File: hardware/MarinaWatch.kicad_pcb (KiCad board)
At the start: 2 copper layers, 82.5 x 100.3 mm, 54 parts, among them J201 USB_C_Receptacle_USB2.0_16P, J401 Screw_Terminal_01x04, J801 Screw_Terminal_01x02, J802 Screw_Terminal_01x03, J803 Screw_Terminal_01x03, U101 ESP32-S3-MINI-1, U301 LMV321, U302 LMV321, U303 LMV321

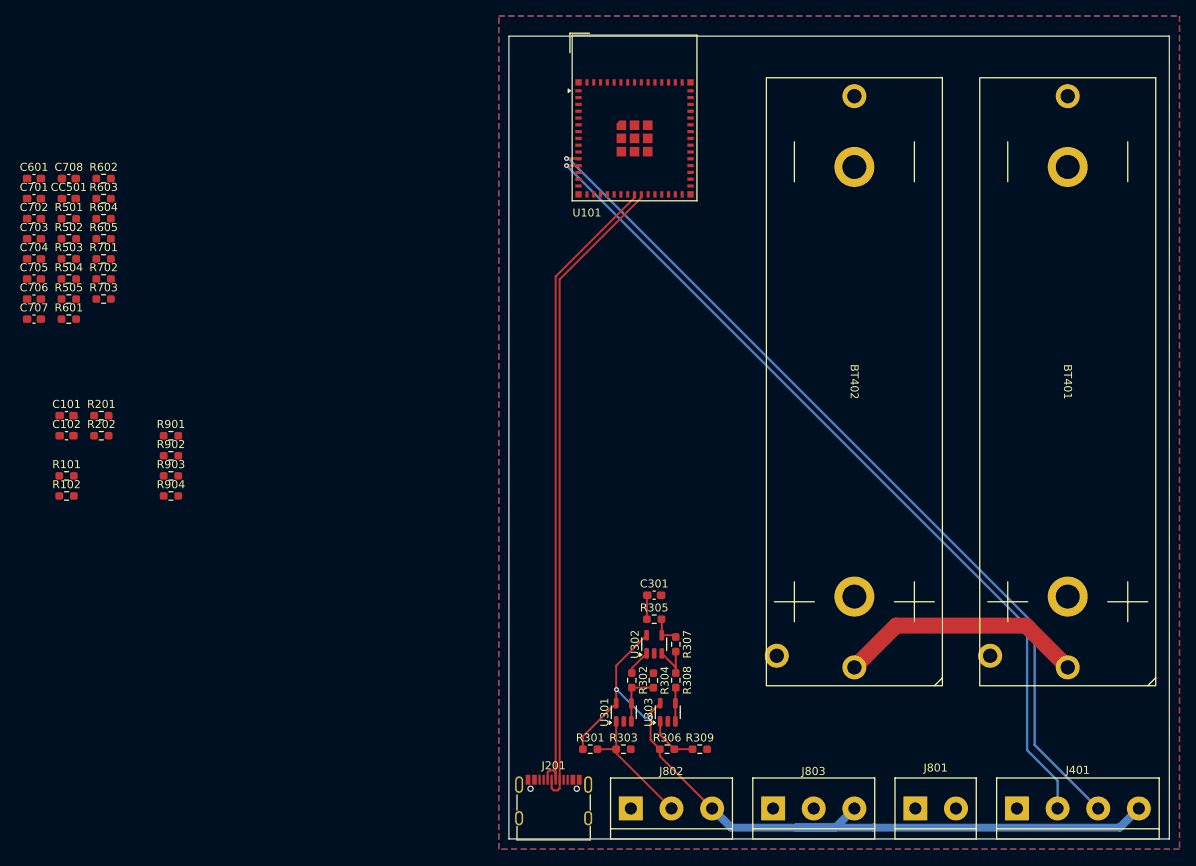
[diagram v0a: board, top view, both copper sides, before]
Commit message: Working on power circuitry layout
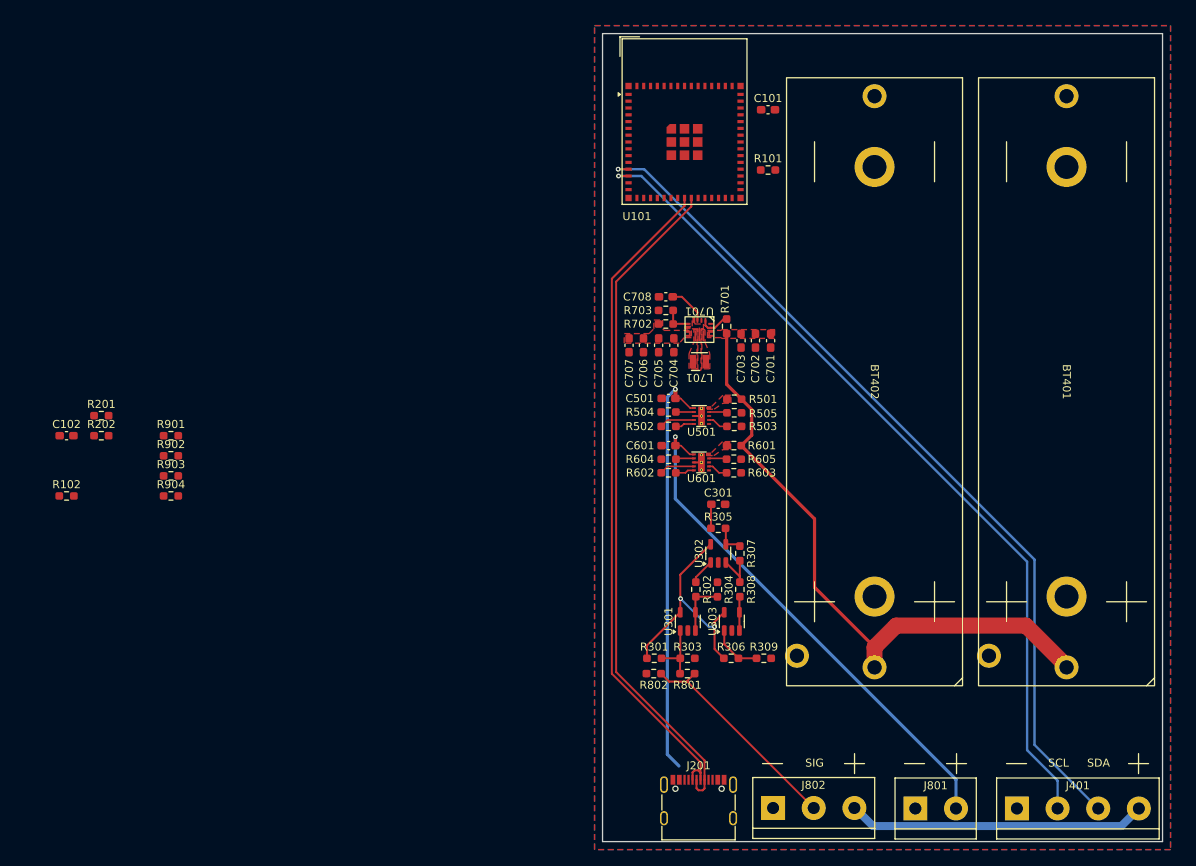
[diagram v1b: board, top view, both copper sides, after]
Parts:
- removed J803: Screw_Terminal_01x03, TerminalBlock:TerminalBlock_bornier-3_P5.08mm
- added L701: 1u5, Inductor_SMD_Wurth:L_Wurth_WE-LQSH-2010, F.Cu at (138.1, 94.0)
- added R801: 100R, Resistor_SMD:R_0603_1608Metric_Pad0.98x0.95mm_HandSolder, F.Cu at (136.6, 133.0)
- added R802: 100R, Resistor_SMD:R_0603_1608Metric_Pad0.98x0.95mm_HandSolder, F.Cu at (132.4, 133.0)
- added U501: BQ24210, AlfredLib:WSON-10, F.Cu at (138.4, 100.8)
- added U601: BQ24210, AlfredLib:WSON-10, F.Cu at (138.4, 106.6)
- added U701: TPS63070, AlfredLib:VQFN-3.0x2.5, F.Cu at (138.1, 90.0)
- moved C101 95.7 mm to (146.7, 62.5)
- moved R101 95.7 mm to (146.7, 70.0)
- moved C701 93.8 mm to (147.0, 91.4), turned to -90 degrees
- moved C702 91.5 mm to (145.1, 91.4), turned to -90 degrees
- moved C703 89.3 mm to (143.3, 91.4), turned to -90 degrees
- moved R501 86.2 mm to (142.5, 98.7)
- moved C601 86.1 mm to (134.2, 104.5), turned to 180 degrees
- moved R603 85.9 mm to (142.4, 107.9)
- moved R503 85.8 mm to (142.5, 102.1)
- moved R601 84.6 mm to (142.4, 104.5)
- moved R505 84.4 mm to (142.5, 100.4)
- moved R605 83.5 mm to (142.4, 106.2)
- moved C704 80.7 mm to (134.9, 92.0), turned to -90 degrees
- moved R602 79.6 mm to (134.2, 107.9)
- moved C501 79.0 mm to (134.2, 98.6), turned to 180 degrees
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- renumbered CC501 to C501
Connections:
- net Net-(U701-FB) renamed /POWER/FB
- C601 pad 2: Net-(U601-VSS) -> GND
- C708 pad 1: Net-(U701-VAUX) -> /POWER/VAUX
- J802 pad 2: /PT100 -> /SIG
- R501 pad 1: Net-(U501-BAT) -> /POWER/USB_BAT
- R502 pad 1: Net-(U501-VTSB) -> /POWER/USB_VTSB
- R502 pad 2: Net-(U501-TS) -> /POWER/USB_TS
- R503 pad 1: Net-(U501-~{EN}) -> /POWER/USB_EN
- R504 pad 1: Net-(U501-ISET) -> /POWER/USB_ISET
- R505 pad 1: Net-(U501-VDPM) -> /POWER/USB_VDPM
- R601 pad 1: Net-(U601-BAT) -> /POWER/SOLAR_BAT
- R602 pad 1: Net-(U601-VTSB) -> /POWER/SOLAR_VTSB
- R602 pad 2: Net-(U601-TS) -> /POWER/SOLAR_TS
- R603 pad 1: Net-(U601-~{EN}) -> /POWER/SOLAR_EN
- R603 pad 2: Net-(U601-VSS) -> GND
- R604 pad 1: Net-(U601-ISET) -> /POWER/SOLAR_ISET
- R604 pad 2: Net-(U601-VSS) -> GND
- R605 pad 1: Net-(U601-VDPM) -> /POWER/SOLAR_VDPM
- R605 pad 2: Net-(U601-VSS) -> GND
- R701 pad 2: Net-(U701-EN) -> /POWER/EN
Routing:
- net SOLAR: track 0.00 -> 64.9 mm, vias 0 -> 1
- net VBUS: track 0.00 -> 52.1 mm, vias 0 -> 1
- net +BATT: track 31.0 -> 79.8 mm
- net +3V3: track 103.7 -> 67.4 mm
- net /SIG: track 0.00 -> 27.5 mm
- net /PT100: track 16.1 -> 7.74 mm
- net /POWER/VAUX: track 0.00 -> 4.90 mm
- net /POWER/USB_VTSB: track 0.00 -> 4.44 mm
- net /POWER/SOLAR_VTSB: track 0.00 -> 4.41 mm
- net /POWER/EN: track 0.00 -> 3.85 mm
- net /D+: track 80.8 -> 84.6 mm
- net /POWER/FB: track 0.00 -> 3.60 mm
- net /D-: track 80.3 -> 83.2 mm
- net /I2C_SCL: track 107.5 -> 104.7 mm
- net /I2C_SDA: track 110.6 -> 108.0 mm
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- added copper zone on F.Cu, net +3V3
- added copper zone on F.Cu, net +BATT
- added copper zone on F.Cu, net /POWER/L1
- added copper zone on F.Cu, net /POWER/L2
- added copper zone on F.Cu, net /POWER/SOLAR_BAT
- added copper zone on F.Cu, net /POWER/USB_BAT
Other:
- board size 82.5 x 100.3 mm -> 70 x 101 mm
- board text added: "SCL"
- board text added: "SDA"
- board text added: "SIG"
